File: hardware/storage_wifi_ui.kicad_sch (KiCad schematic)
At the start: 29 parts, among them J16 Keyboard KIN0-7 / KOUT0-7, J17 Keyboard power/reference, J18 I2C0, J19 Full-size SD, SPI, J20 ESP-01/ESP-01S socket, J36 MicroSD alternative, SPI, SW2 ESP_PROG, U34 AMS1117-3.3

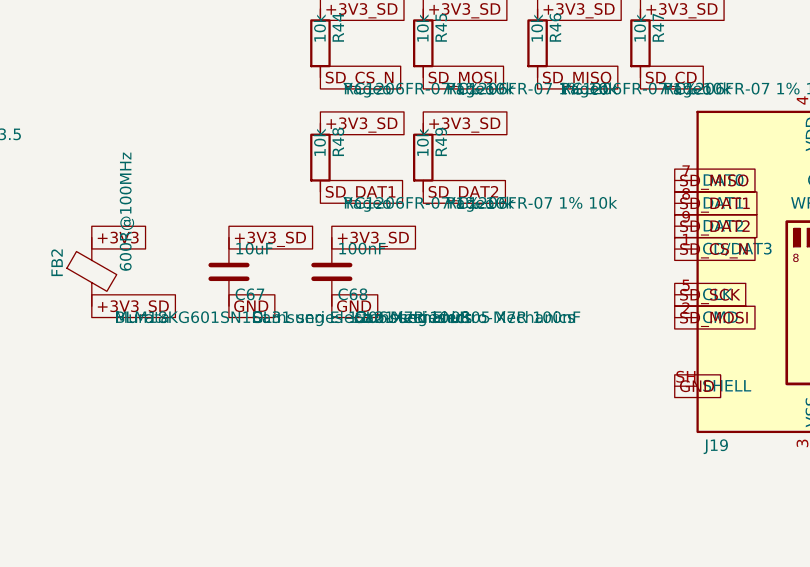
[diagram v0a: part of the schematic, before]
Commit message: BOM simplification
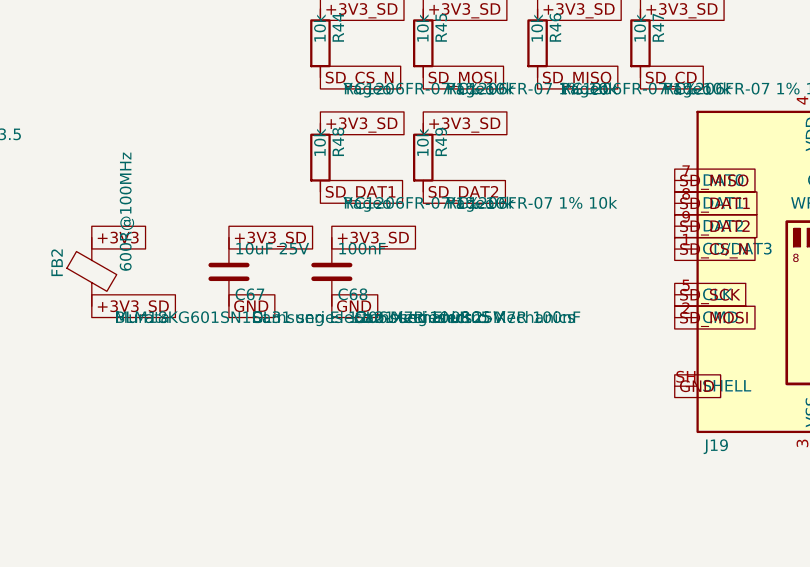
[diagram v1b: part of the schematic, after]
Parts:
- C67: value 10uF -> 10uF 25V; MPN CL31 series 1206 X7R 10uF -> CL31 series 1206 X7R 10uF 25V
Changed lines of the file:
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@@
 		(instances
 			(project "Storage, Wi-Fi and UI"
-				(path "/9f4f8ddb-6d75-424f-85af-50d3b0c33d12"
+				(path "/ebd1e8ca-9dff-4053-89c8-43c30a776960"
 					(reference "J16")
 					(unit 1)
@@
 		(instances
 			(project "Storage, Wi-Fi and UI"
-				(path "/9f4f8ddb-6d75-424f-85af-50d3b0c33d12"
+				(path "/ebd1e8ca-9dff-4053-89c8-43c30a776960"
 					(reference "J17")
 					(unit 1)
@@
 		(instances
 			(project "Storage, Wi-Fi and UI"
-				(path "/9f4f8ddb-6d75-424f-85af-50d3b0c33d12"
+				(path "/ebd1e8ca-9dff-4053-89c8-43c30a776960"
 					(reference "RN22")
 					(unit 1)
@@
 		(instances
 			(project "Storage, Wi-Fi and UI"
-				(path "/9f4f8ddb-6d75-424f-85af-50d3b0c33d12"
+				(path "/ebd1e8ca-9dff-4053-89c8-43c30a776960"
 					(reference "RN24")
 					(unit 1)
@@
 		(instances
 			(project "Storage, Wi-Fi and UI"
-				(path "/9f4f8ddb-6d75-424f-85af-50d3b0c33d12"
+				(path "/ebd1e8ca-9dff-4053-89c8-43c30a776960"
 					(reference "J18")
 					(unit 1)
@@
 		(instances
 			(project "Storage, Wi-Fi and UI"
-				(path "/9f4f8ddb-6d75-424f-85af-50d3b0c33d12"
+				(path "/ebd1e8ca-9dff-4053-89c8-43c30a776960"
 					(reference "J19")
 					(unit 1)
@@
 		(instances
 			(project "Storage, Wi-Fi and UI"
-				(path "/9f4f8ddb-6d75-424f-85af-50d3b0c33d12"
+				(path "/ebd1e8ca-9dff-4053-89c8-43c30a776960"
 					(reference "R44")
 					(unit 1)
@@
 		(instances
 			(project "Storage, Wi-Fi and UI"
-				(path "/9f4f8ddb-6d75-424f-85af-50d3b0c33d12"
+				(path "/ebd1e8ca-9dff-4053-89c8-43c30a776960"
 					(reference "R45")
 					(unit 1)
@@
 		(instances
 			(project "Storage, Wi-Fi and UI"
-				(path "/9f4f8ddb-6d75-424f-85af-50d3b0c33d12"
+				(path "/ebd1e8ca-9dff-4053-89c8-43c30a776960"
 					(reference "R46")
 					(unit 1)
@@
 		(instances
 			(project "Storage, Wi-Fi and UI"
-				(path "/9f4f8ddb-6d75-424f-85af-50d3b0c33d12"
+				(path "/ebd1e8ca-9dff-4053-89c8-43c30a776960"
 					(reference "R47")
 					(unit 1)
@@
 		(instances
 			(project "Storage, Wi-Fi and UI"
-				(path "/9f4f8ddb-6d75-424f-85af-50d3b0c33d12"
+				(path "/ebd1e8ca-9dff-4053-89c8-43c30a776960"
 					(reference "R48")
 					(unit 1)
@@
 		(instances
 			(project "Storage, Wi-Fi and UI"
-				(path "/9f4f8ddb-6d75-424f-85af-50d3b0c33d12"
+				(path "/ebd1e8ca-9dff-4053-89c8-43c30a776960"
 					(reference "R49")
 					(unit 1)
@@
 		(instances
 			(project "Storage, Wi-Fi and UI"
-				(path "/9f4f8ddb-6d75-424f-85af-50d3b0c33d12"
+				(path "/ebd1e8ca-9dff-4053-89c8-43c30a776960"
 					(reference "R50")
 					(unit 1)
@@
 		(instances
 			(project "Storage, Wi-Fi and UI"
-				(path "/9f4f8ddb-6d75-424f-85af-50d3b0c33d12"
+				(path "/ebd1e8ca-9dff-4053-89c8-43c30a776960"
 					(reference "R51")
 					(unit 1)
@@
 		(instances
 			(project "Storage, Wi-Fi and UI"
-				(path "/9f4f8ddb-6d75-424f-85af-50d3b0c33d12"
+				(path "/ebd1e8ca-9dff-4053-89c8-43c30a776960"
 					(reference "R52")
 					(unit 1)
@@
 		(instances
 			(project "Storage, Wi-Fi and UI"
-				(path "/9f4f8ddb-6d75-424f-85af-50d3b0c33d12"
+				(path "/ebd1e8ca-9dff-4053-89c8-43c30a776960"
 					(reference "R53")
 					(unit 1)
@@
 		(instances
 			(project "Storage, Wi-Fi and UI"
-				(path "/9f4f8ddb-6d75-424f-85af-50d3b0c33d12"
+				(path "/ebd1e8ca-9dff-4053-89c8-43c30a776960"
 					(reference "FB2")
 					(unit 1)
@@
 			)
 		)
-		(property "Value" "10uF"
+		(property "Value" "10uF 25V"
 			(at 90.805 167.64 0.0000)
 			(effects
@@
 			)
 		)
-		(property "MPN" "CL31 series 1206 X7R 10uF"
+		(property "MPN" "CL31 series 1206 X7R 10uF 25V"
 			(at 92.71 175.2599 0)
 			(effects
@@
 		(instances
 			(project "Storage, Wi-Fi and UI"
-				(path "/9f4f8ddb-6d75-424f-85af-50d3b0c33d12"
+				(path "/ebd1e8ca-9dff-4053-89c8-43c30a776960"
 					(reference "C67")
 					(unit 1)
@@
 		(instances
 			(project "Storage, Wi-Fi and UI"
-				(path "/9f4f8ddb-6d75-424f-85af-50d3b0c33d12"
+				(path "/ebd1e8ca-9dff-4053-89c8-43c30a776960"
 					(reference "C68")
 					(unit 1)
@@
 		(instances
 			(project "Storage, Wi-Fi and UI"
-				(path "/9f4f8ddb-6d75-424f-85af-50d3b0c33d12"
+				(path "/ebd1e8ca-9dff-4053-89c8-43c30a776960"
 					(reference "JP5")
 					(unit 1)
@@
 		(instances
 			(project "Storage, Wi-Fi and UI"
-				(path "/9f4f8ddb-6d75-424f-85af-50d3b0c33d12"
+				(path "/ebd1e8ca-9dff-4053-89c8-43c30a776960"
 					(reference "J20")
 					(unit 1)
@@
 		(instances
 			(project "Storage, Wi-Fi and UI"
-				(path "/9f4f8ddb-6d75-424f-85af-50d3b0c33d12"
+				(path "/ebd1e8ca-9dff-4053-89c8-43c30a776960"
 					(reference "SW2")
 					(unit 1)
@@
 		(instances
 			(project "Storage, Wi-Fi and UI"
-				(path "/9f4f8ddb-6d75-424f-85af-50d3b0c33d12"
+				(path "/ebd1e8ca-9dff-4053-89c8-43c30a776960"
 					(reference "C69")
 					(unit 1)
@@
 		(instances
 			(project "Storage, Wi-Fi and UI"
-				(path "/9f4f8ddb-6d75-424f-85af-50d3b0c33d12"
+				(path "/ebd1e8ca-9dff-4053-89c8-43c30a776960"
 					(reference "C70")
 					(unit 1)
@@
 		(instances
 			(project "Storage, Wi-Fi and UI"
-				(path "/9f4f8ddb-6d75-424f-85af-50d3b0c33d12"
+				(path "/ebd1e8ca-9dff-4053-89c8-43c30a776960"
 					(reference "U34")
 					(unit 1)
@@
 		(instances
 			(project "Storage, Wi-Fi and UI"
-				(path "/9f4f8ddb-6d75-424f-85af-50d3b0c33d12"
+				(path "/ebd1e8ca-9dff-4053-89c8-43c30a776960"
 					(reference "C88")
 					(unit 1)
@@
 		(instances
 			(project "Storage, Wi-Fi and UI"
-				(path "/9f4f8ddb-6d75-424f-85af-50d3b0c33d12"
+				(path "/ebd1e8ca-9dff-4053-89c8-43c30a776960"
 					(reference "C89")
 					(unit 1)
@@
 		(instances
 			(project "Storage, Wi-Fi and UI"
-				(path "/9f4f8ddb-6d75-424f-85af-50d3b0c33d12"
+				(path "/ebd1e8ca-9dff-4053-89c8-43c30a776960"
 					(reference "RN36")
 					(unit 1)
@@
 		(instances
 			(project "Storage, Wi-Fi and UI"
-				(path "/9f4f8ddb-6d75-424f-85af-50d3b0c33d12"
+				(path "/ebd1e8ca-9dff-4053-89c8-43c30a776960"
 					(reference "J36")
 					(unit 1)
